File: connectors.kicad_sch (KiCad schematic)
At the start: 37 parts, among them J2 Pyro Channels, J3 Screw Switches, J4 JST-PH, J6 Serial Wire Debug, J7 USB_C_Receptacle_USB2.0, J8 External UART, J9 External I2C, Q10 AO3401A, Q9 AO3401A, U2 USBLC6-2SC6, U8 TPS61230DRC, U9 LM3670MF

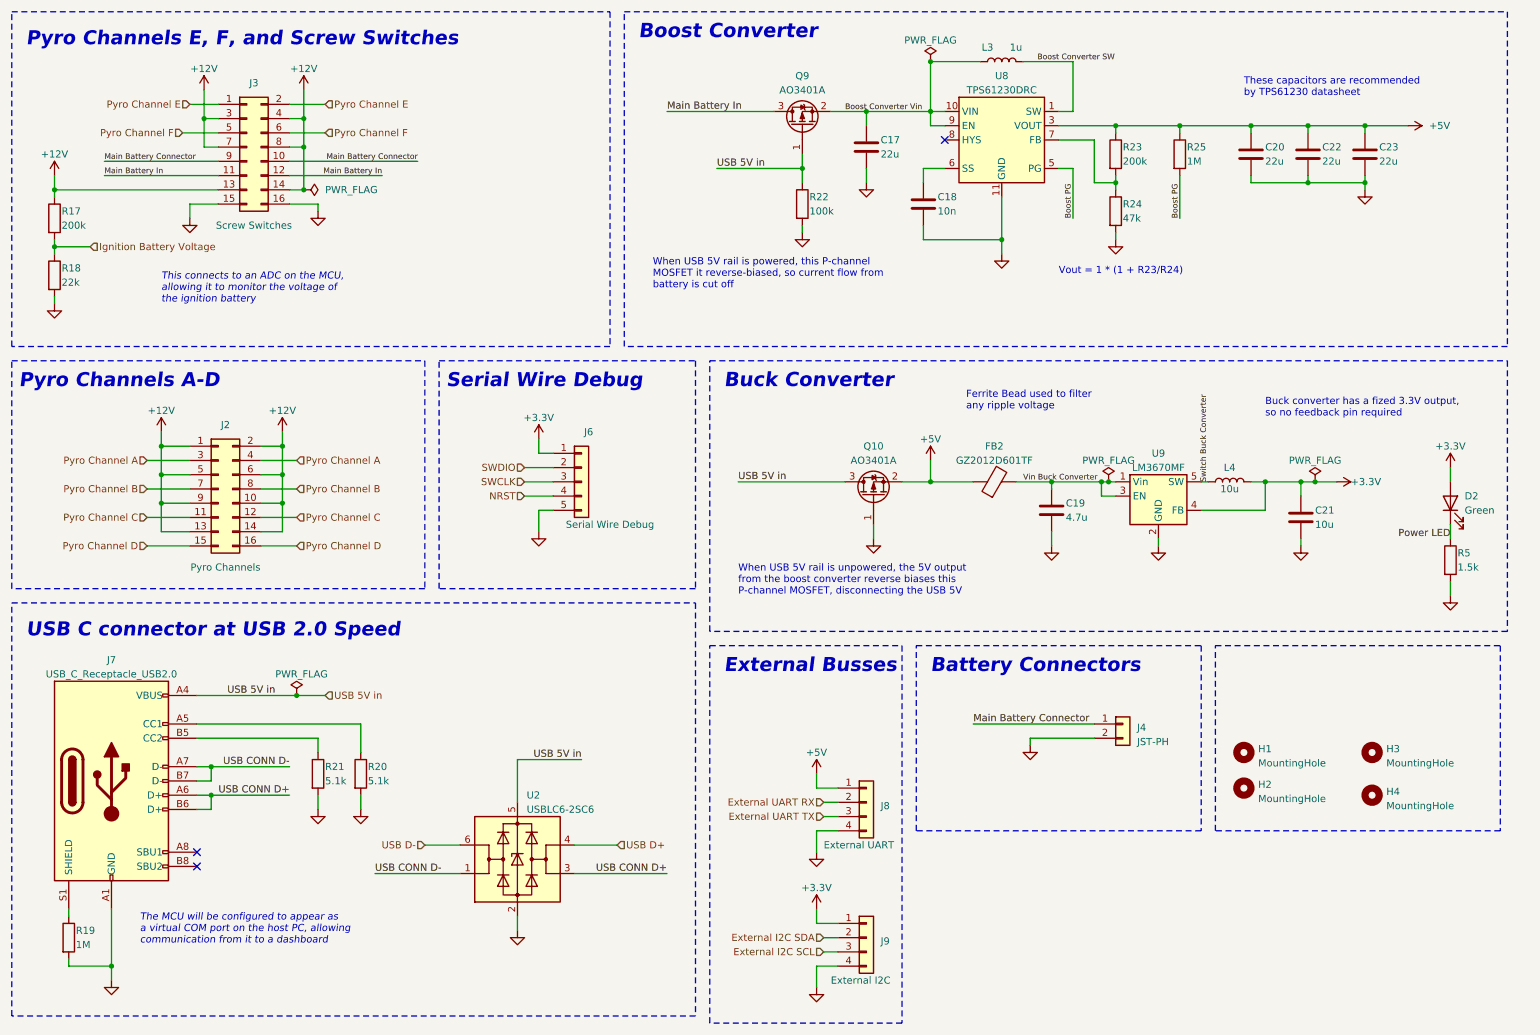
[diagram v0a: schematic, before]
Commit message: How many sheets do you want? Yes
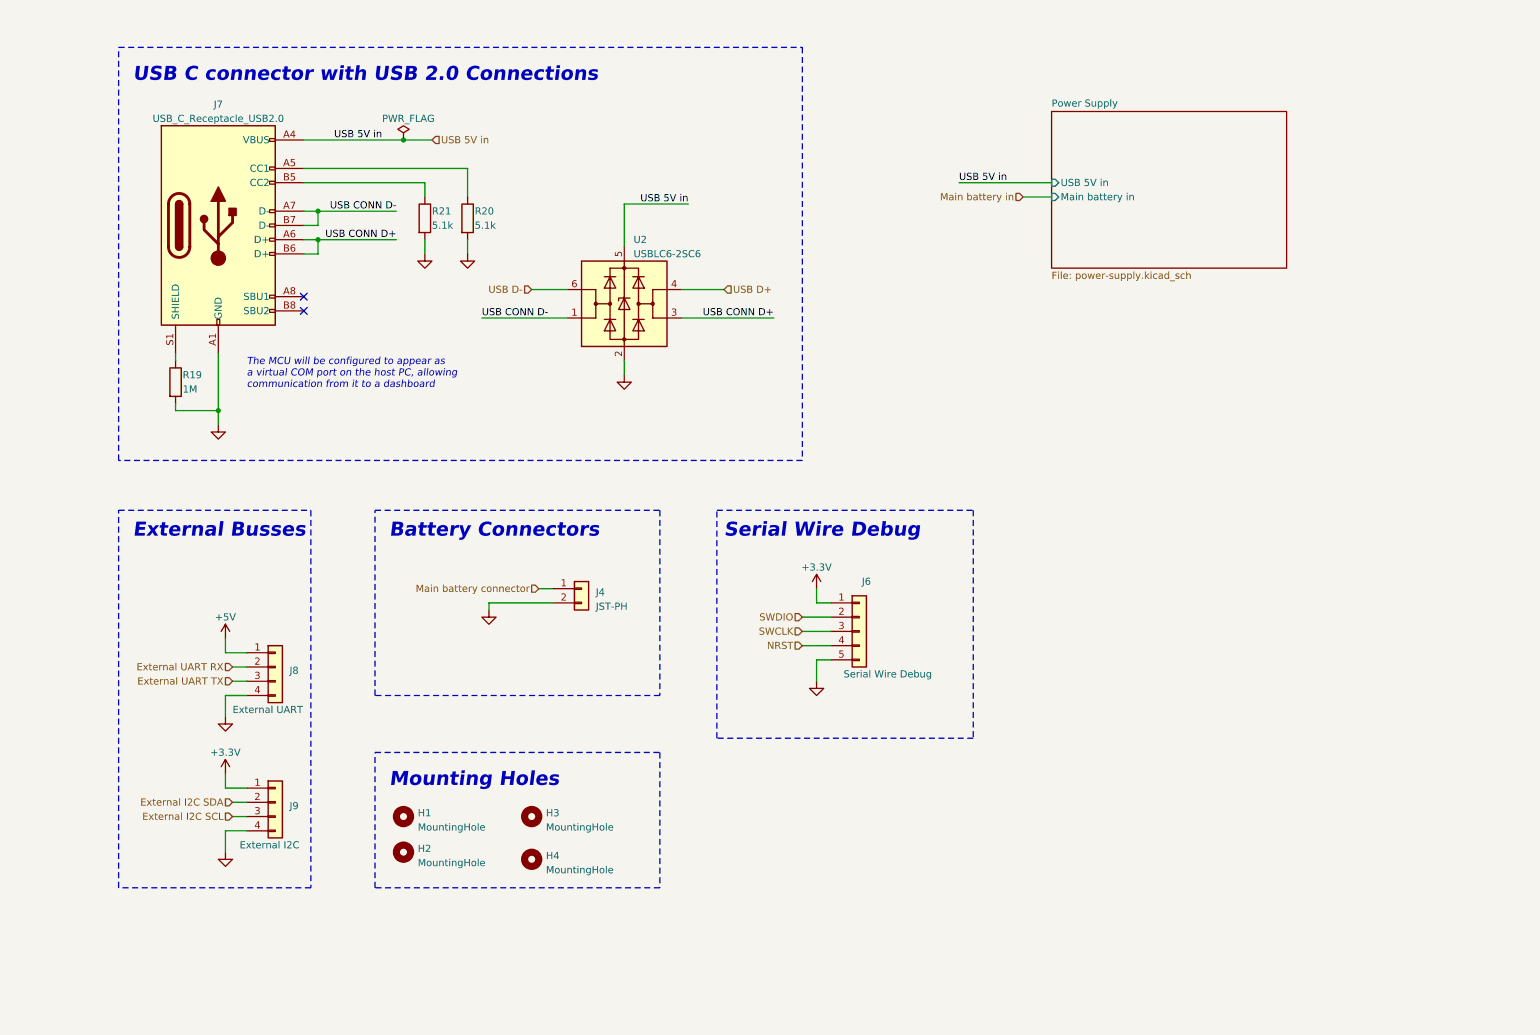
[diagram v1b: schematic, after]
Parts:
- removed C17, C20, C22, C23: 22u, Capacitor_SMD:C_0805_2012Metric, symbol Device:C
- removed C18: 10n, Capacitor_SMD:C_0402_1005Metric, symbol Device:C
- removed C19: 4.7u, Capacitor_SMD:C_0603_1608Metric, symbol Device:C
- removed C21: 10u, Capacitor_SMD:C_0805_2012Metric, symbol Device:C
- removed D2: Green, LED_SMD:LED_0805_2012Metric, symbol Device:LED
- removed FB2: GZ2012D601TF, Inductor_SMD:L_0805_2012Metric, symbol Device:FerriteBead
- removed J2: Pyro Channels, custom-footprints:Wago_Custom_218-108, symbol Connector_Generic:Conn_02x08_Odd_Even
- removed J3: Screw Switches, custom-footprints:Wago_Custom_218-108, symbol Connector_Generic:Conn_02x08_Odd_Even
- removed L3: 1u, Inductor_SMD:L_Sunlord_SWPA4030S, symbol Device:L
- removed L4: 10u, Inductor_SMD:L_Sunlord_SWPA4030S, symbol Device:L
- removed Q10, Q9: AO3401A, Package_TO_SOT_SMD:SOT-23, symbol Transistor_FET:AO3401A
- removed R17, R23: 200k, Resistor_SMD:R_0402_1005Metric, symbol Device:R
- removed R18: 22k, Resistor_SMD:R_0402_1005Metric, symbol Device:R
- removed R22: 100k, Resistor_SMD:R_0402_1005Metric, symbol Device:R
- removed R24: 47k, Resistor_SMD:R_0402_1005Metric, symbol Device:R
- removed R25: 1M, Resistor_SMD:R_0402_1005Metric, symbol Device:R
- removed R5: 1.5k, Resistor_SMD:R_0603_1608Metric, symbol Device:R
- removed U8: TPS61230DRC, Package_SON:Texas_S-PVSON-N10_ThermalVias, symbol Regulator_Switching:TPS61230DRC
- removed U9: LM3670MF, Package_TO_SOT_SMD:TSOT-23-5, symbol Regulator_Switching:LM3670MF
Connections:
- net Main Battery Connector renamed Main battery connector
- no-connect marks 3 -> 2
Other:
- added sheet Power Supply (power-supply.kicad_sch)
- note added: "Mounting Holes"
- note added: "USB C connector with USB 2.0 Connections"
- note removed: "Boost Converter"
- note removed: "Buck Converter"
- note removed: "Buck converter has a fized 3.3V output, so no feedback pin required"
- note removed: "Ferrite Bead used to filter any ripple voltage"
- note removed: "Pyro Channels A-D"
- note removed: "Pyro Channels E, F, and Screw Switches"
- note removed: "These capacitors are recommended by TPS61230 datasheet"
- note removed: "This connects to an ADC on the MCU, allowing it to monitor the voltage of the ignition battery"
- note removed: "USB C connector at USB 2.0 Speed"
- note removed: "Vout = 1 * (1 + R23/R24)"
- note removed: "When USB 5V rail is powered, this P-channel MOSFET it reverse-biased, so current flow from battery is cut off"
- note removed: "When USB 5V rail is unpowered, the 5V output from the boost converter reverse biases this P-channel MOSFET, disconnecting the USB 5V"
- moved on the sheet: H1, H2, H3, H4, J4, J6, J7, J8, J9, R19, R20, R21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

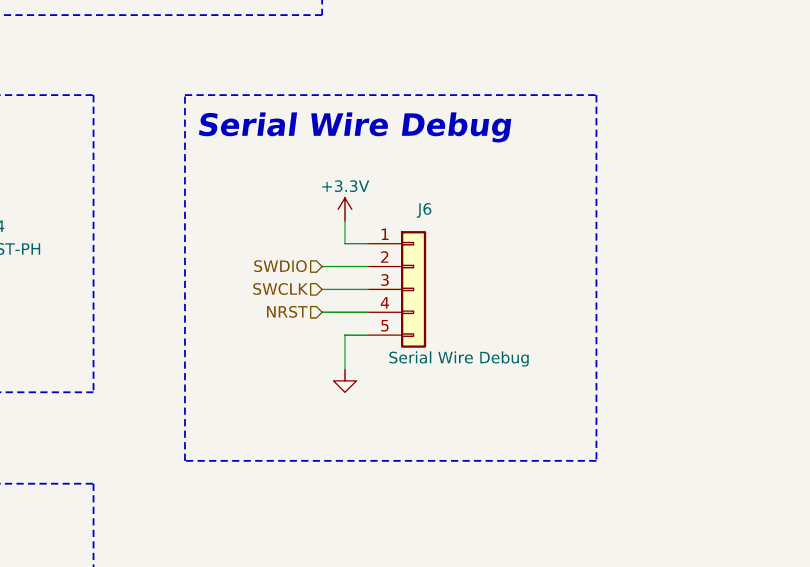
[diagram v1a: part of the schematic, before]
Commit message: finished layout for v1.1
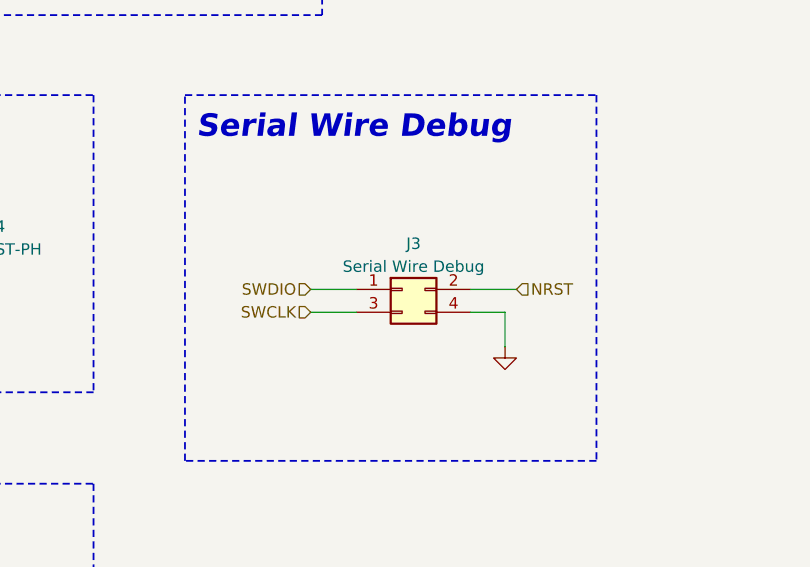
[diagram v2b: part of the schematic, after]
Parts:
- removed J6: Serial Wire Debug, Connector_PinHeader_2.54mm:PinHeader_1x05_P2.54mm_Vertical, symbol Connector_Generic:Conn_01x05
- added J3: Serial Wire Debug, Connector_PinHeader_2.54mm:PinHeader_2x02_P2.54mm_Vertical, symbol Connector_Generic:Conn_02x02_Odd_Even
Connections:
- net GND: now also J3.4 (Pin_4)
- net NRST: now also J3.2 (Pin_2)
- net SWCLK: now also J3.3 (Pin_3)
- net SWDIO: now also J3.1 (Pin_1)
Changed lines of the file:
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@@
     (stroke (width 0) (type default))
   )
-  (wire (pts (xy 161.29 123.19) (xy 156.21 123.19))
+  (wire (pts (xy 160.02 125.73) (xy 154.94 125.73))
     (stroke (width 0) (type default))
   )
@@
     (stroke (width 0) (type default))
   )
-  (wire (pts (xy 158.75 130.81) (xy 158.75 134.62))
+  (wire (pts (xy 176.53 128.27) (xy 176.53 132.08))
     (stroke (width 0) (type default))
   )
@@
     (stroke (width 0) (type default))
   )
-  (wire (pts (xy 158.75 130.81) (xy 161.29 130.81))
-    (stroke (width 0) (type default))
-  )
-  (wire (pts (xy 156.21 128.27) (xy 161.29 128.27))
+  (wire (pts (xy 176.53 128.27) (xy 172.72 128.27))
+    (stroke (width 0) (type default))
+  )
+  (wire (pts (xy 177.8 125.73) (xy 172.72 125.73))
     (stroke (width 0) (type default))
   )
@@
     (stroke (width 0) (type default))
   )
-  (wire (pts (xy 161.29 120.65) (xy 158.75 120.65))
-    (stroke (width 0) (type default))
-  )
   (wire (pts (xy 195.58 48.26) (xy 200.66 48.26))
     (stroke (width 0) (type default))
@@
     (stroke (width 0) (type default))
   )
-  (wire (pts (xy 156.21 125.73) (xy 161.29 125.73))
+  (wire (pts (xy 154.94 128.27) (xy 160.02 128.27))
     (stroke (width 0) (type default))
   )
@@
   )
   (wire (pts (xy 96.52 55.88) (xy 96.52 58.42))
-    (stroke (width 0) (type default))
-  )
-  (wire (pts (xy 158.75 118.11) (xy 158.75 120.65))
     (stroke (width 0) (type default))
   )
@@
     (effects (font (size 1.27 1.27)) (justify right))
   )
-  (hierarchical_label "SWCLK" (shape input) (at 156.21 125.73 180) (fields_autoplaced)
+  (hierarchical_label "SWCLK" (shape input) (at 154.94 128.27 180) (fields_autoplaced)
     (effects (font (size 1.27 1.27)) (justify right))
   )
@@
     (effects (font (size 1.27 1.27)) (justify right))
   )
-  (hierarchical_label "SWDIO" (shape input) (at 156.21 123.19 180) (fields_autoplaced)
+  (hierarchical_label "SWDIO" (shape input) (at 154.94 125.73 180) (fields_autoplaced)
     (effects (font (size 1.27 1.27)) (justify right))
   )
@@
     (effects (font (size 1.27 1.27)) (justify left))
   )
-  (hierarchical_label "NRST" (shape input) (at 156.21 128.27 180) (fields_autoplaced)
-    (effects (font (size 1.27 1.27)) (justify right))
+  (hierarchical_label "NRST" (shape input) (at 177.8 125.73 0) (fields_autoplaced)
+    (effects (font (size 1.27 1.27)) (justify left))
   )
   (hierarchical_label "Main battery connector" (shape input) (at 109.22 118.11 180) (fields_autoplaced)
@@
     )
   )
-  (symbol (lib_id "power:+3.3V") (at 158.75 118.11 0) (unit 1)
-    (in_bom yes) (on_board yes) (dnp no) (fields_autoplaced)
-    (property "Reference" "#PWR050" (at 158.75 121.92 0)
-      (effects (font (size 1.27 1.27)) hide)
-    )
-    (property "Value" "+3.3V" (at 158.75 114.3 0)
-      (effects (font (size 1.27 1.27)))
-    )
-    (property "Footprint" "" (at 158.75 118.11 0)
-      (effects (font (size 1.27 1.27)) hide)
-    )
-    (property "Datasheet" "" (at 158.75 118.11 0)
-      (effects (font (size 1.27 1.27)) hide)
-    )
-    (pin "1")
-    (instances
-      (project "Flight Computer"
-        (path "/0c1188a1-706b-46cd-a73a-5b3f8187d77a/afc466af-6d84-4e19-b5b5-aea43618ea20"
-          (reference "#PWR050") (unit 1)
-        )
-      )
-    )
-  )
   (symbol (lib_id "Connector_Generic:Conn_01x04") (at 62.23 132.08 0) (unit 1)
     (in_bom yes) (on_board yes) (dnp no)
@@
     )
   )
-  (symbol (lib_id "power:GND") (at 158.75 134.62 0) (unit 1)
-    (in_bom yes) (on_board yes) (dnp no) (fields_autoplaced)
-    (property "Reference" "#PWR051" (at 158.75 140.97 0)
-      (effects (font (size 1.27 1.27)) hide)
-    )
-    (property "Value" "GND" (at 158.75 139.7 0)
-      (effects (font (size 1.27 1.27)) hide)
-    )
-    (property "Footprint" "" (at 158.75 134.62 0)
-      (effects (font (size 1.27 1.27)) hide)
-    )
-    (property "Datasheet" "" (at 158.75 134.62 0)
+  (symbol (lib_id "power:GND") (at 176.53 132.08 0) (unit 1)
+    (in_bom yes) (on_board yes) (dnp no)
+    (property "Reference" "#PWR051" (at 176.53 138.43 0)
+      (effects (font (size 1.27 1.27)) hide)
+    )
+    (property "Value" "GND" (at 176.53 137.16 0)
+      (effects (font (size 1.27 1.27)) hide)
+    )
+    (property "Footprint" "" (at 176.53 132.08 0)
+      (effects (font (size 1.27 1.27)) hide)
+    )
+    (property "Datasheet" "" (at 176.53 132.08 0)
       (effects (font (size 1.27 1.27)) hide)
     )
@@
         (path "/0c1188a1-706b-46cd-a73a-5b3f8187d77a/afc466af-6d84-4e19-b5b5-aea43618ea20"
           (reference "#PWR059") (unit 1)
-        )
-      )
-    )
-  )
-  (symbol (lib_id "Connector_Generic:Conn_01x05") (at 166.37 125.73 0) (unit 1)
-    (in_bom yes) (on_board yes) (dnp no)
-    (property "Reference" "J6" (at 167.64 116.84 0)
-      (effects (font (size 1.27 1.27)))
-    )
-    (property "Value" "Serial Wire Debug" (at 171.45 133.35 0)
-      (effects (font (size 1.27 1.27)))
-    )
-    (property "Footprint" "Connector_PinHeader_2.54mm:PinHeader_1x05_P2.54mm_Vertical" (at 166.37 125.73 0)
-      (effects (font (size 1.27 1.27)) hide)
-    )
-    (property "Datasheet" "~" (at 166.37 125.73 0)
-      (effects (font (size 1.27 1.27)) hide)
-    )
-    (pin "1")
-    (pin "2")
-    (pin "3")
-    (pin "4")
-    (pin "5")
-    (instances
-      (project "Flight Computer"
-        (path "/0c1188a1-706b-46cd-a73a-5b3f8187d77a/afc466af-6d84-4e19-b5b5-aea43618ea20"
-          (reference "J6") (unit 1)
         )
       )
@@
         )
       )
+    )
+  )
+  (symbol (lib_id "Connector_Generic:Conn_02x02_Odd_Even") (at 165.1 125.73 0) (unit 1)
+    (in_bom yes) (on_board yes) (dnp no) (fields_autoplaced)
+    (property "Reference" "J3" (at 166.37 120.65 0)
+      (effects (font (size 1.27 1.27)))
+    )
+    (property "Value" "Serial Wire Debug" (at 166.37 123.19 0)
+      (effects (font (size 1.27 1.27)))
+    )
+    (property "Footprint" "Connector_PinHeader_2.54mm:PinHeader_2x02_P2.54mm_Vertical" (at 165.1 125.73 0)
+      (effects (font (size 1.27 1.27)) hide)
+    )
+    (property "Datasheet" "~" (at 165.1 125.73 0)
+      (effects (font (size 1.27 1.27)) hide)
+    )
+    (pin "1")
+    (pin "2")
+    (pin "3")
+    (pin "4")
+    (instances
+      (project "Flight Computer"
+        (path "/0c1188a1-706b-46cd-a73a-5b3f8187d77a/afc466af-6d84-4e19-b5b5-aea43618ea20"
+          (reference "J3") (unit 1)
+        )
+      )
